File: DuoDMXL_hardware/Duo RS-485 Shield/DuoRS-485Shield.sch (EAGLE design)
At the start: 15 parts, among them IC1 SN65176PS

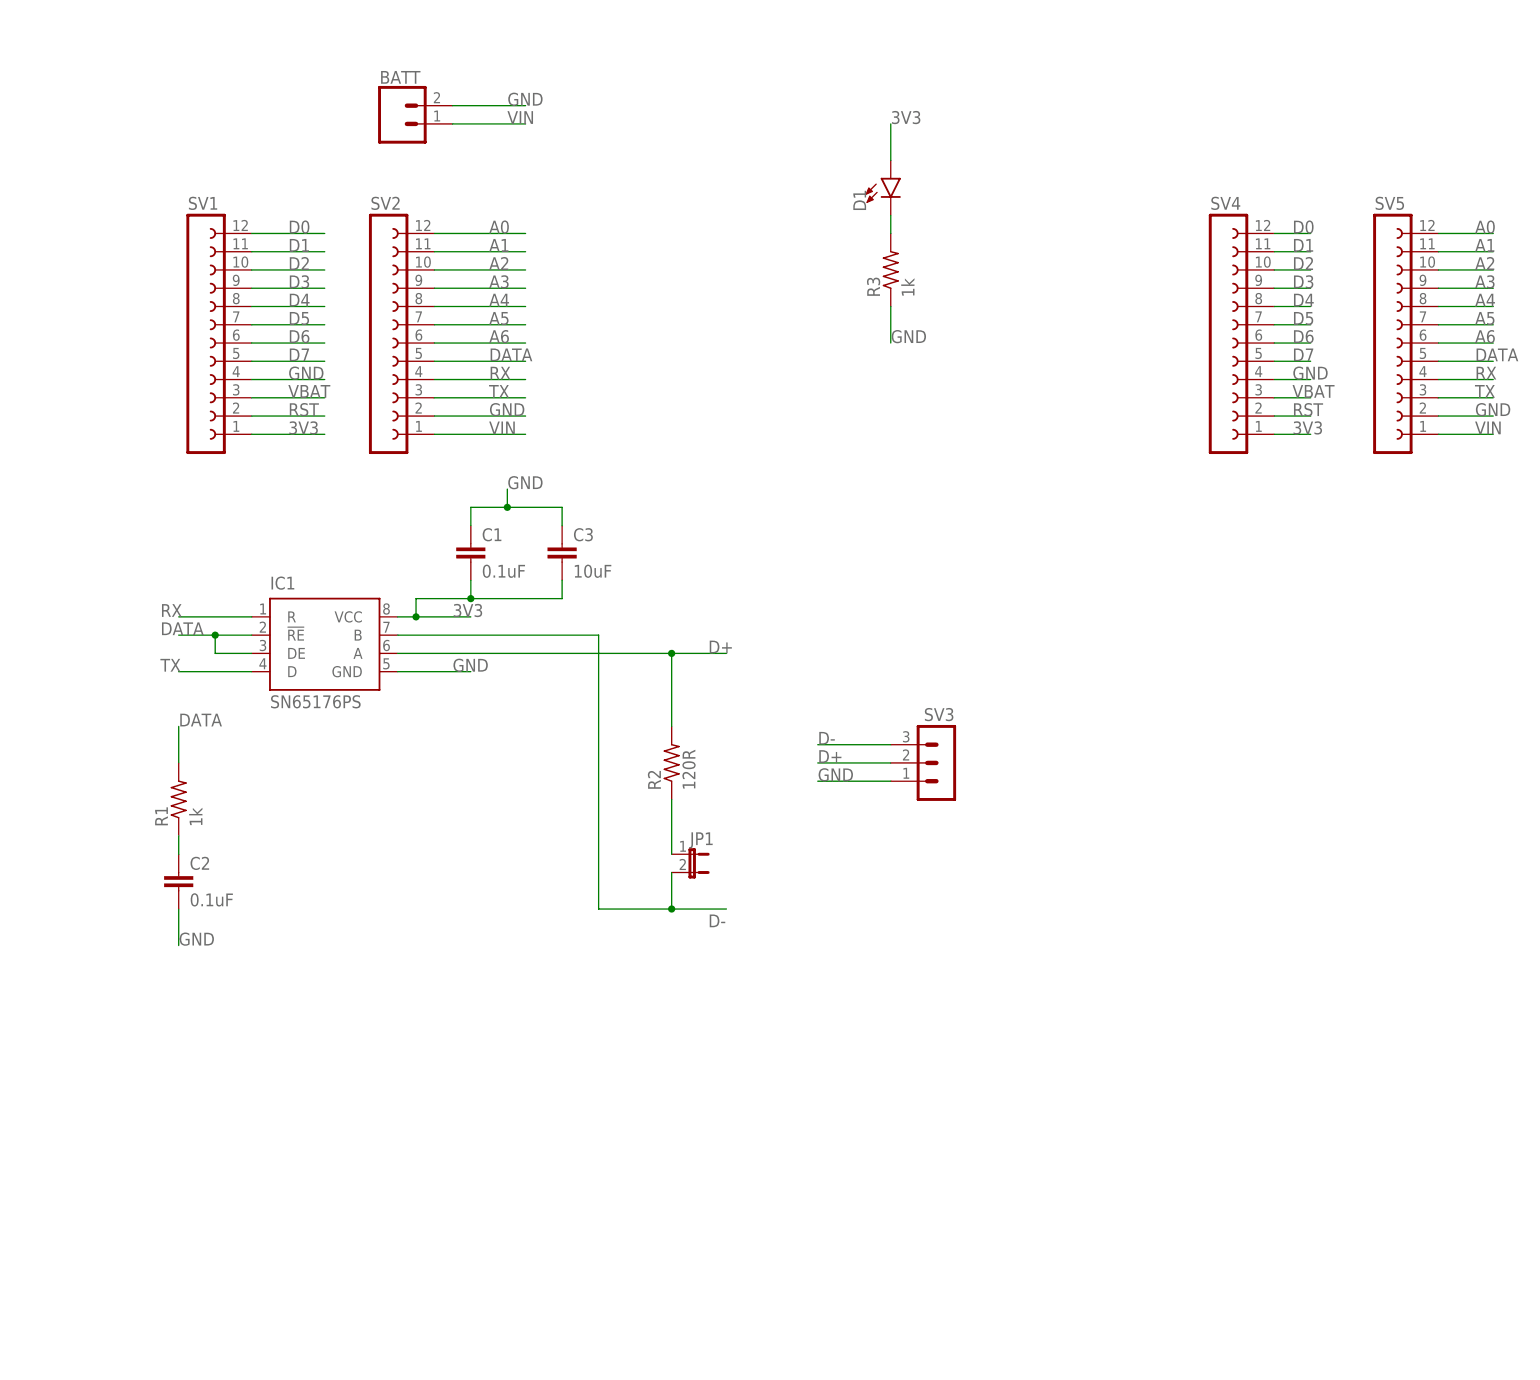
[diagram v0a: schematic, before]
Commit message: Add .gitignore
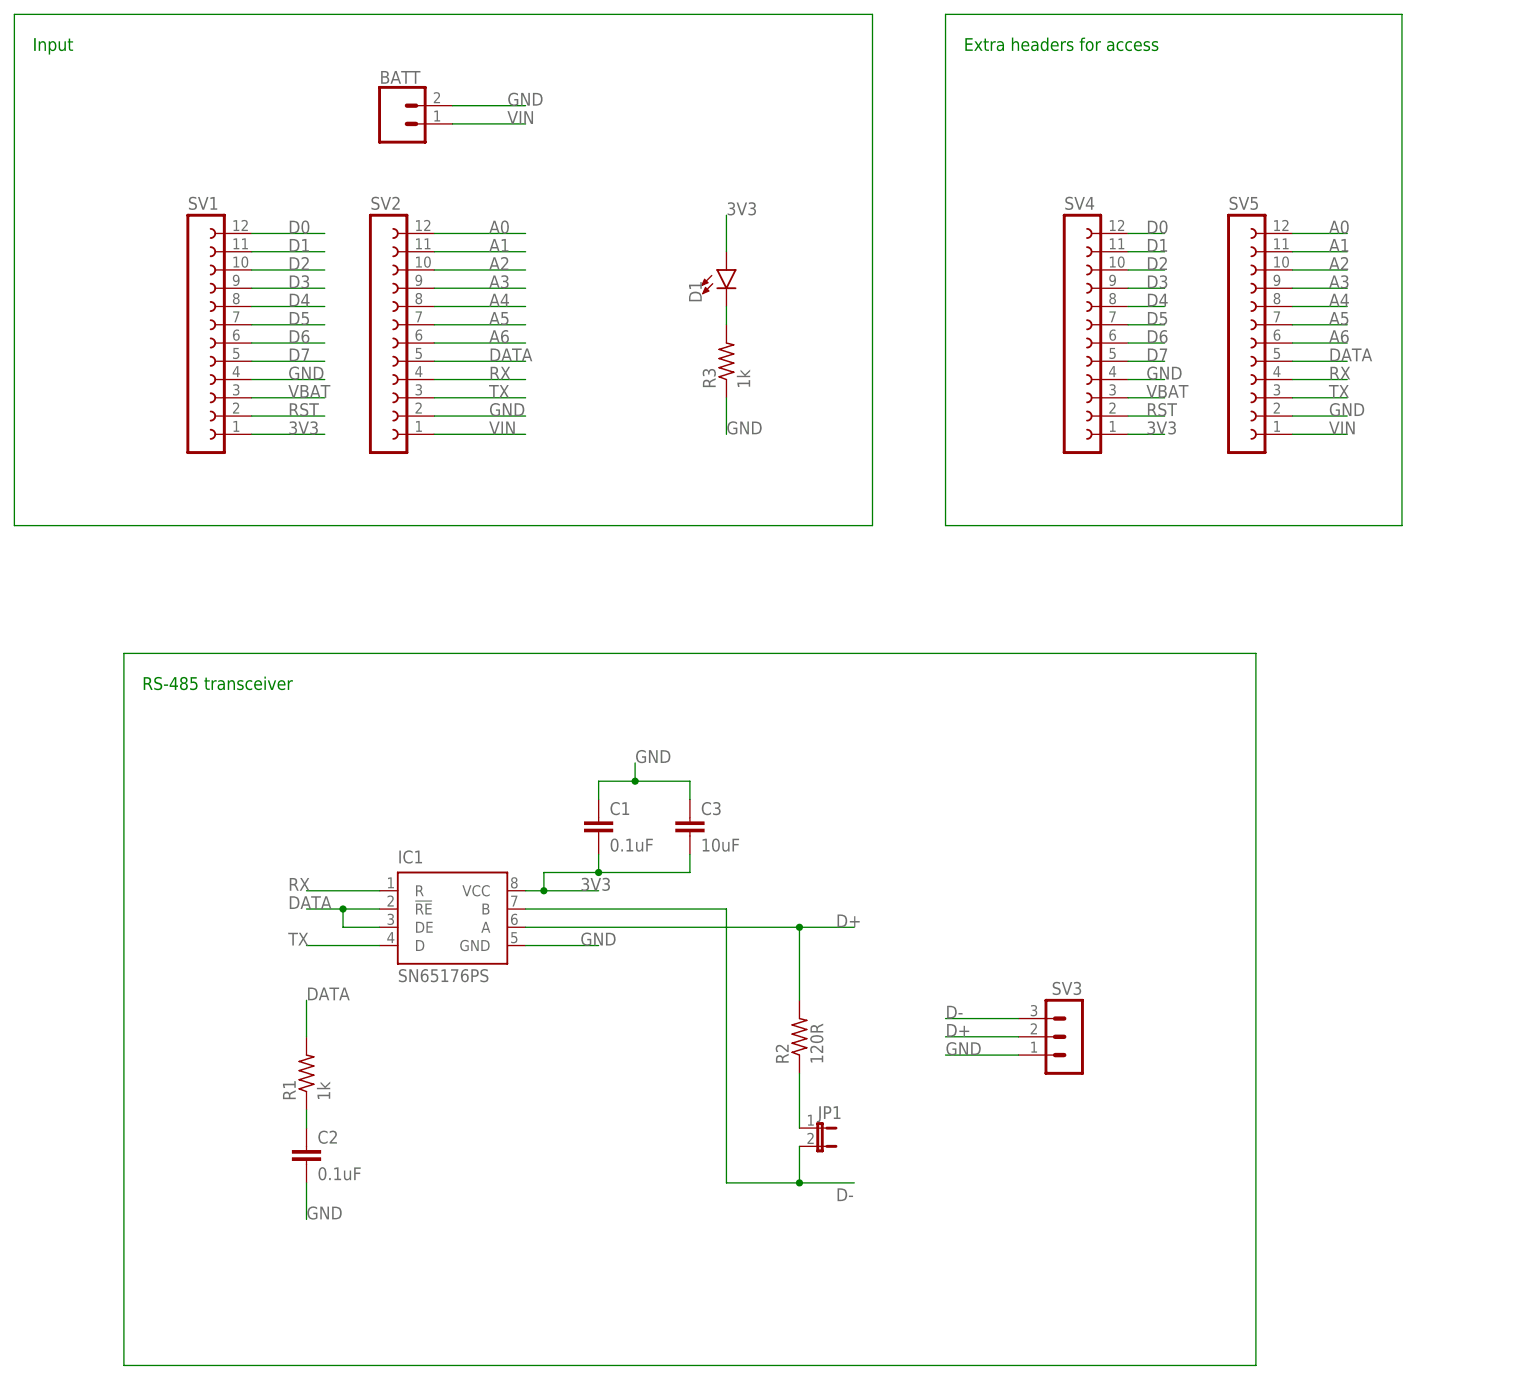
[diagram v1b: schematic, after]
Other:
- note added: "Extra headers for access"
- note added: "Input"
- note added: "RS-485 transceiver"
- moved on the sheet: C1, C2, C3, D1, IC1, JP1, R1, R2, R3, SV3, SV4, SV5
